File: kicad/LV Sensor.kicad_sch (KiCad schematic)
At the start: 70 parts, among them J16 USB_B_Micro, SW1 SW_Push, U1 AP63205WU-7, U10 LM2662MX/NOPB, U2 XMSM0C1104SPW20R, U3 FT231XS-R, U4 AP63203WU-7, U5 TLV77325PDBVR, U6 MCP2518FD-xJHA, U7 DSC1001DL5-020.0000T, U8 ADS114S06BIPBSR, U9 ATA6561-GAQW-N

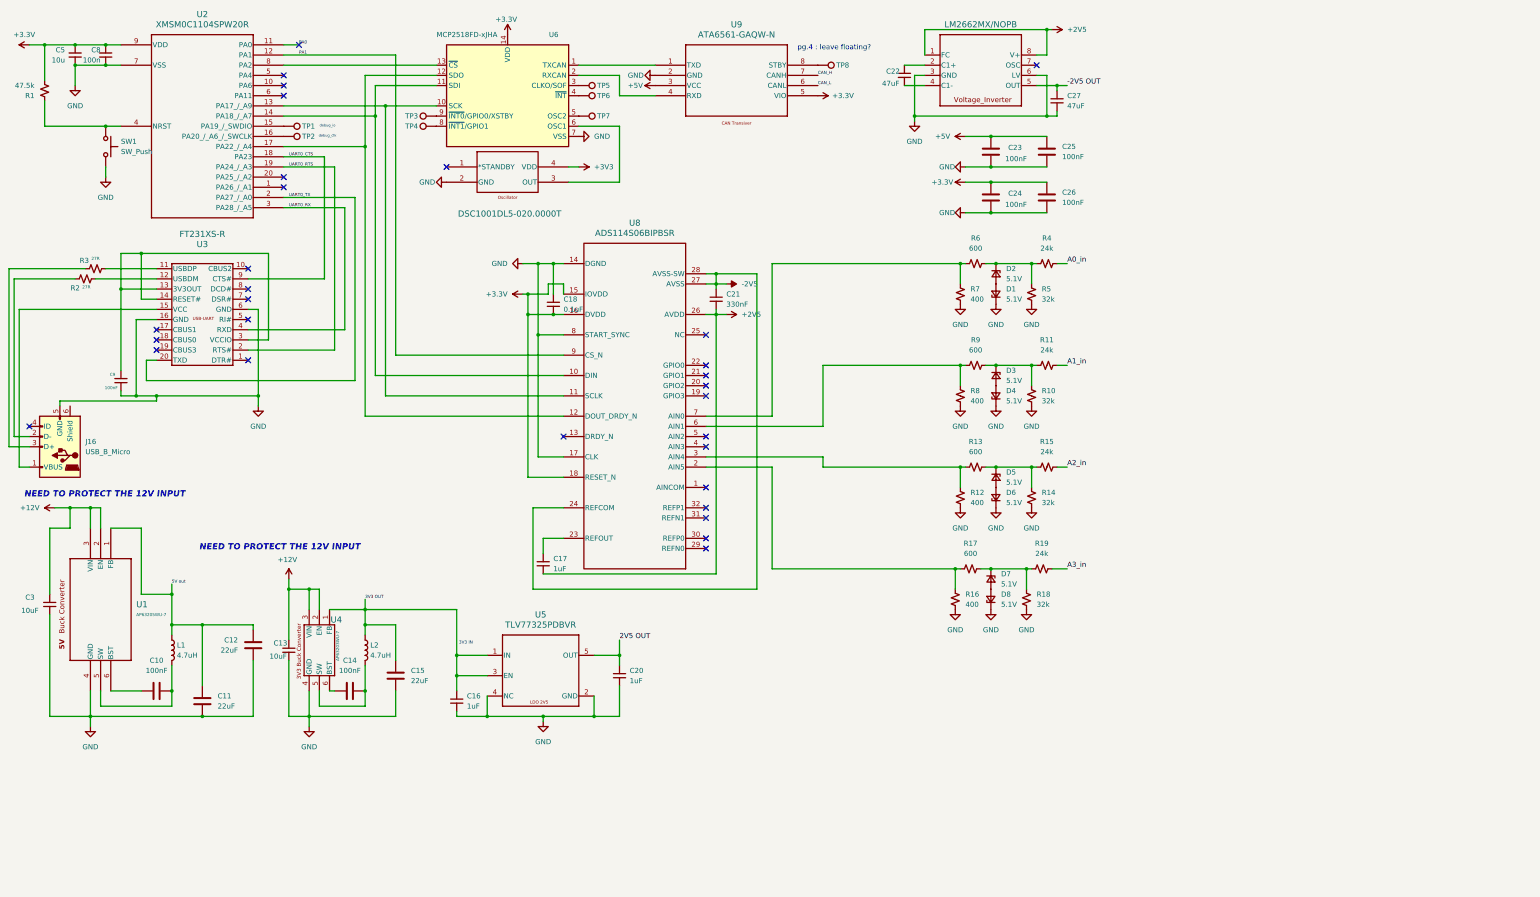
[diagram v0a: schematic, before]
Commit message: aerg
Completely fixed everything

Co-Authored-By: Manish Shrestha <manish.shr006@gmail.com>
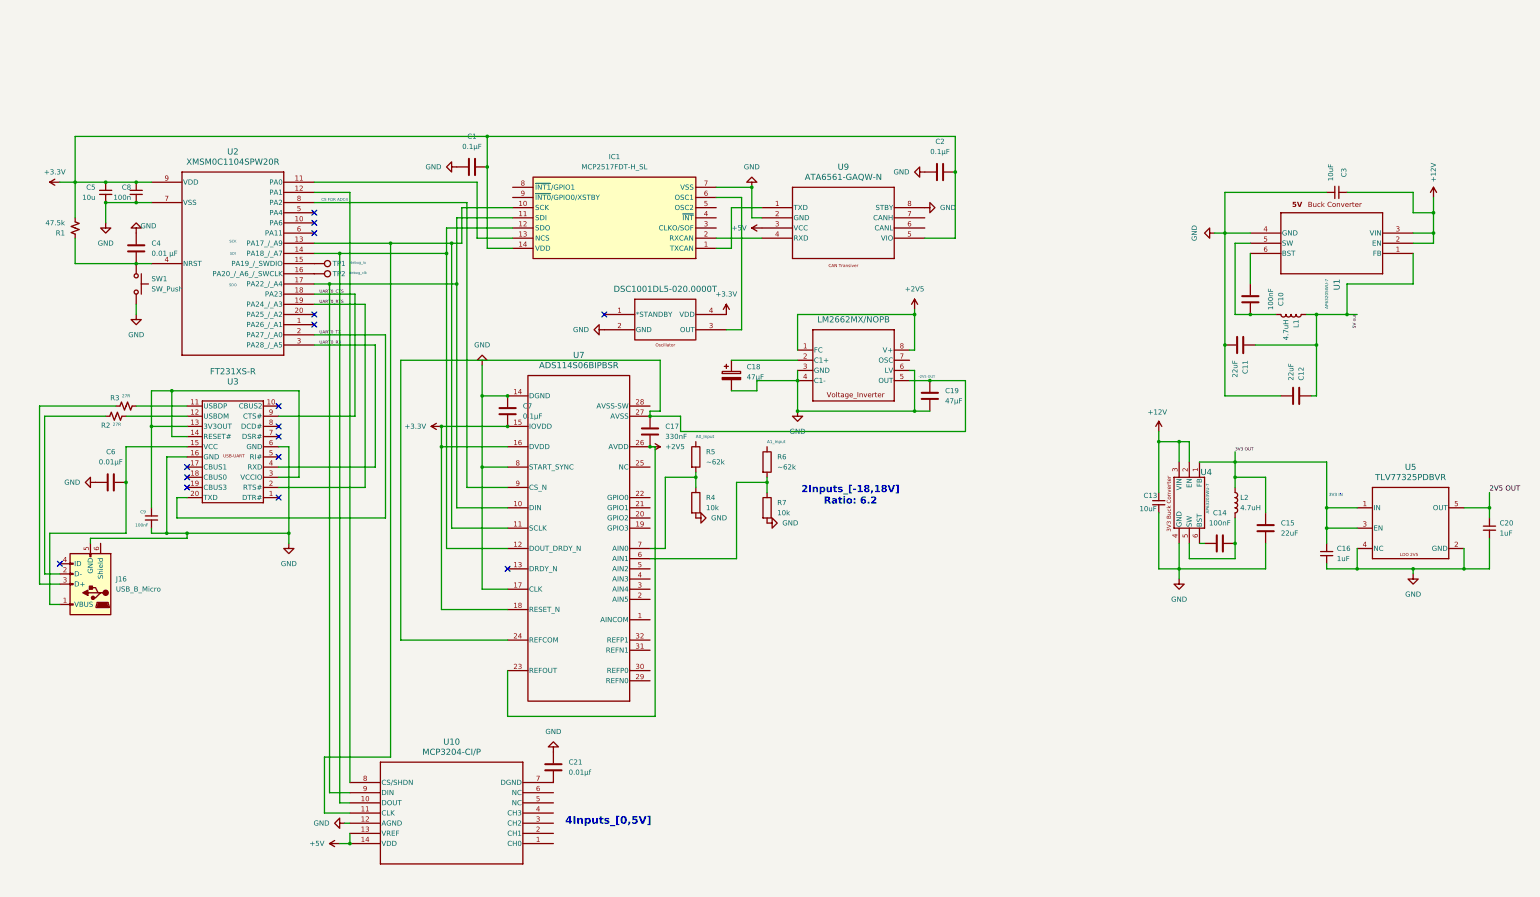
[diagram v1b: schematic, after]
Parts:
- removed C17: 1uF, Capacitor_SMD:C_1206_3216Metric_Pad1.33x1.80mm_HandSolder, symbol Device:C_Small
- removed C18: 0.1uF, Capacitor_SMD:C_1206_3216Metric_Pad1.33x1.80mm_HandSolder, symbol Device:C_Small
- removed C21: 330nF, Capacitor_SMD:C_1206_3216Metric_Pad1.33x1.80mm_HandSolder, symbol Device:C_Small
- removed C22, C27: 47uF, Capacitor_SMD:C_1206_3216Metric_Pad1.33x1.80mm_HandSolder, symbol Device:C_Small
- removed C23, C24, C25, C26: 100nF, Capacitor_SMD:C_1206_3216Metric_Pad1.33x1.80mm_HandSolder, symbol Device:C
- removed D1, D2, D3, D4, D5, D6, D7, D8: 5.1V, symbol Device:D_Zener_Small
- removed R10, R14, R18, R5: 32k, symbol Device:R_Small_US
- removed R11, R15, R19, R4: 24k, symbol Device:R_Small_US
- removed R12, R16, R7, R8: 400, symbol Device:R_Small_US
- removed R13, R17, R6, R9: 600, symbol Device:R_Small_US
- removed TP3, TP4, TP5, TP6, TP7, TP8: TestPoint, symbol Connector:TestPoint
- removed U10: LM2662MX/NOPB, LV-Sensor-Footprints-Lib:M08A, symbol LV-Sensor-Lib:LM2662MX_NOPB
- removed U6: MCP2518FD-xJHA, LV-Sensor-Footprints-Lib:MCP2518FDT, symbol LV-Sensor-Lib:MCP2517FD-xJHA
- removed U7: DSC1001DL5-020.0000T, LV-Sensor-Footprints-Lib:CDFN4_2P5X2_MCH, symbol LV-Sensor-Lib:DSC1001DL5-020.0000T
- removed U8: ADS114S06BIPBSR, LV-Sensor-Footprints-Lib:PBS0032A_N, symbol LV-Sensor-Lib:ADS114S06BIPBSR
- added C1, C2, C7: 0.1µF, symbol Device:C
- added C17: 330nF, symbol Device:C
- added C18: 47µF, symbol Device:C_Polarized
- added C19: 47µF, symbol Device:C
- added C21: 0.01µf, symbol Device:C
- added C4: 0.01 µF, symbol Device:C
- added C6: 0.01µF, symbol Device:C
- added IC1: MCP2517FDT-H_SL, SOIC127P600X175-14N, symbol CANFDControllerNew:MCP2517FDT-H_SL
- added R4, R7: 10k, symbol Device:R
- added R5, R6: ~62k, symbol Device:R
- added U10: MCP3204-CI/P, PDIP14_300MC_MCH, symbol ADC4Channel:MCP3204-CI_P
- added U6: DSC1001DL5-020.0000T, LV-Sensor-Footprints-Lib:CDFN4_2P5X2_MCH, symbol LV-Sensor-Lib:DSC1001DL5-020.0000T
- added U7: ADS114S06BIPBSR, LV-Sensor-Footprints-Lib:PBS0032A_N, symbol LV-Sensor-Lib:ADS114S06BIPBSR
- added U8: LM2662MX/NOPB, LV-Sensor-Footprints-Lib:M08A, symbol LV-Sensor-Lib:LM2662MX_NOPB
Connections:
- net +2V5: now also C17.2, U7.23 (REFOUT), U7.26 (AVDD), U8.1 (FC), U8.8 (V+)
- net +3.3V: now also C1.2, C2.2, C7.2, IC1.14 (VDD), U6.4 (VDD), U7.15 (IOVDD), U7.16 (DVDD), U7.18 (RESET_N)
- net +5V: now also U10.13 (VREF), U10.14 (VDD)
- net GND: now also U9.8 (STBY), C1.1, C18.2, C19.2, C2.1, C21.1, C4.1, C6.1, C7.1, IC1.7 (VSS), R4.2, R7.2, U10.12 (AGND), U6.2 (GND), U7.14 (DGND), U7.17 (CLK), U7.8 (START_SYNC), U8.3 (GND), U8.4 (C1-), U8.6 (LV)
- net at J16.1 (VBUS), U3.15 (VCC): now also C6.2
- net at U2.14 (PA18_/_A7): now also IC1.12 (SDO), U10.10 (DOUT), U7.12 (DOUT_DRDY_N)
- net at U2.13 (PA17_/_A9): now also IC1.10 (SCK), U10.11 (CLK), U7.11 (SCLK)
- net at U2.17 (PA22_/_A4): now also IC1.11 (SDI), U10.9 (DIN), U7.10 (DIN)
- net at U9.1 (TXD): now also IC1.1 (TXCAN)
- net at U9.4 (RXD): now also IC1.2 (RXCAN)
- net at R1.1, SW1.1, U2.4 (NRST): now also C4.2
- net at U2.8 (PA2): now also U7.9 (CS_N)
- net CAN_H: no longer names the net of U9.7 (CANH)
- net CAN_L: no longer names the net of U9.6 (CANL)
- net PA0: no longer names the net of U2.11 (PA0)
- net PA0: now also IC1.13 (NCS)
- net PA1: no longer names the net of U2.12 (PA1)
- net PA1: now also U10.8 (CS/SHDN)
- new net: C17.1, C19.1, U7.24 (REFCOM), U7.27 (AVSS), U8.5 (OUT)
- new net: IC1.6 (OSC1), U6.3 (OUT)
- new net: R6.2, R7.1, U7.6 (AIN1)
- new net: R4.1, R5.2, U7.7 (AIN0)
- new net: C18.1, U8.2 (C1+)
- new net: C21.2, U10.7 (DGND)
- no-connect marks 30 -> 16
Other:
- note added: "-2V5 OUT"
- note added: "2Inputs_[-18,18V] Ratio: 6.2"
- note added: "4Inputs_[0,5V]"
- note added: "A0_Input"
- note added: "A1_Input"
- note added: "CS FOR ADC4"
- note added: "SCK"
- note added: "SDI"
- note added: "SDO"
- note removed: "NEED TO PROTECT THE 12V INPUT"
- note removed: "pg.4 : leave floating?"
- moved on the sheet: C10, C11, C12, C13, C14, C15, C16, C20, C3, C5, C8, C9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

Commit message: rgwg
fixxes
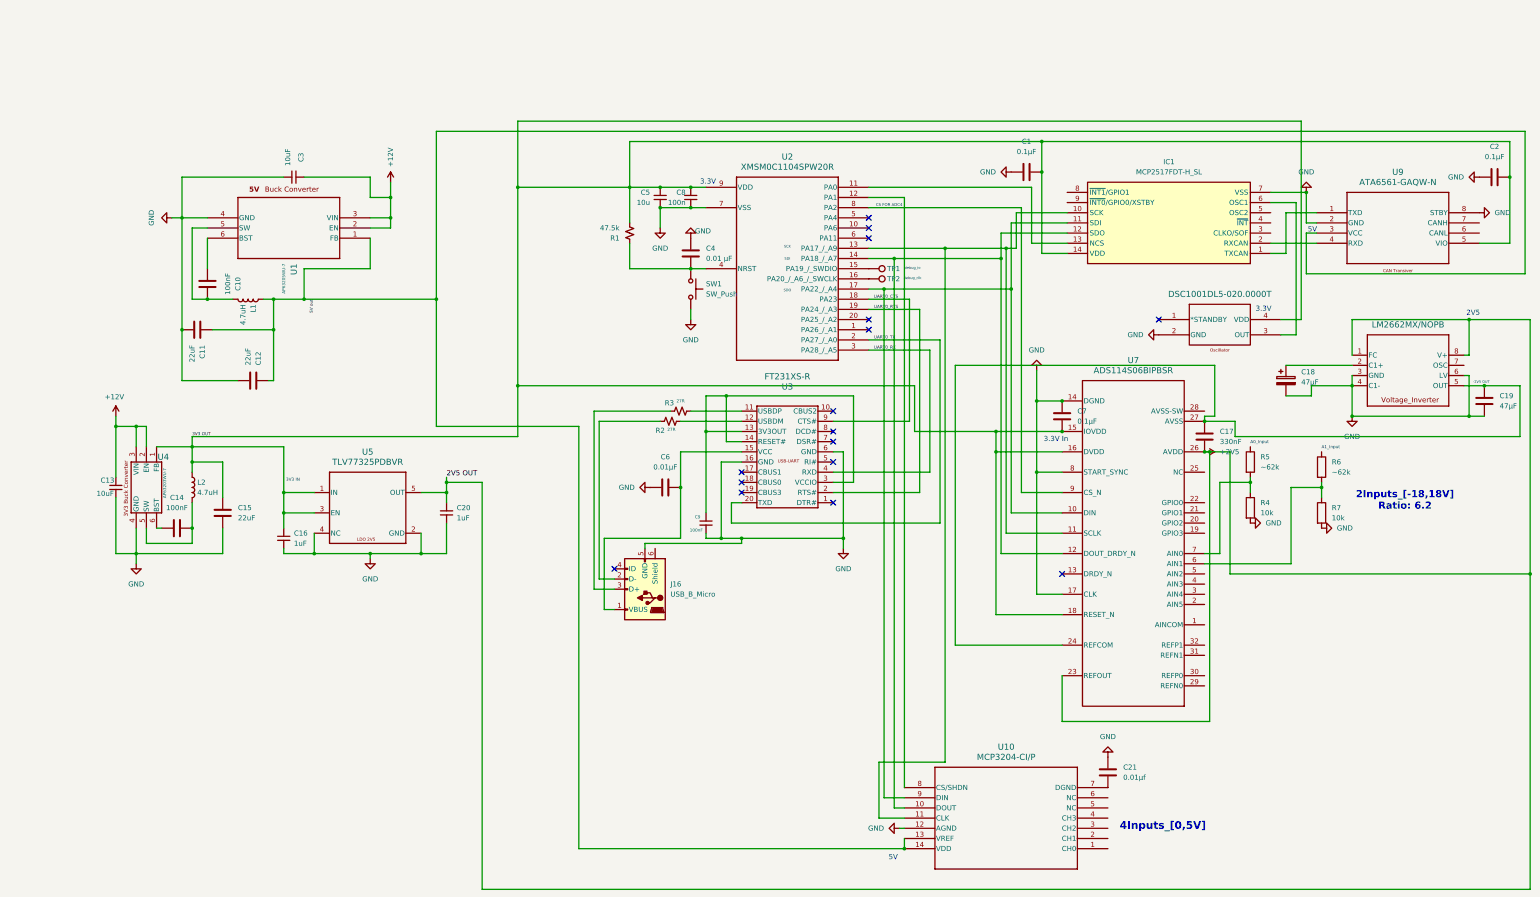
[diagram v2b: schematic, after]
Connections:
- net +3.3V is gone; now on net 3V3 OUT: C1.2, C2.2, C5.1, C7.2, C8.1, IC1.14 (VDD), R1.2, U2.9 (VDD), U6.4 (VDD), U7.15 (IOVDD), U7.16 (DVDD), U7.18 (RESET_N), U9.5 (VIO)
- net +5V is gone; now on net 5V out: U10.13 (VREF), U10.14 (VDD), U9.3 (VCC)
- net 2V5 OUT is gone; now on net +2V5: C20.1, U5.5 (OUT)
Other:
- note added: "2V5"
- note added: "3.3V"
- note added: "3.3V In"
- note added: "5V"
- moved on the sheet: C1, C10, C11, C12, C13, C14, C15, C16, C17, C18, C19, C2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
